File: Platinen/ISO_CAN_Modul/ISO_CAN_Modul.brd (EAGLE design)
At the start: 35.1 x 27.9 mm, 26 parts, among them CON8 Term, IC1 MCP2515-I/P, IC2 ISO1050, IC3 B0505S-1W, X1 8 MHz, X2 Male, X3 Male, X4 Male, X5 AK500/2+M

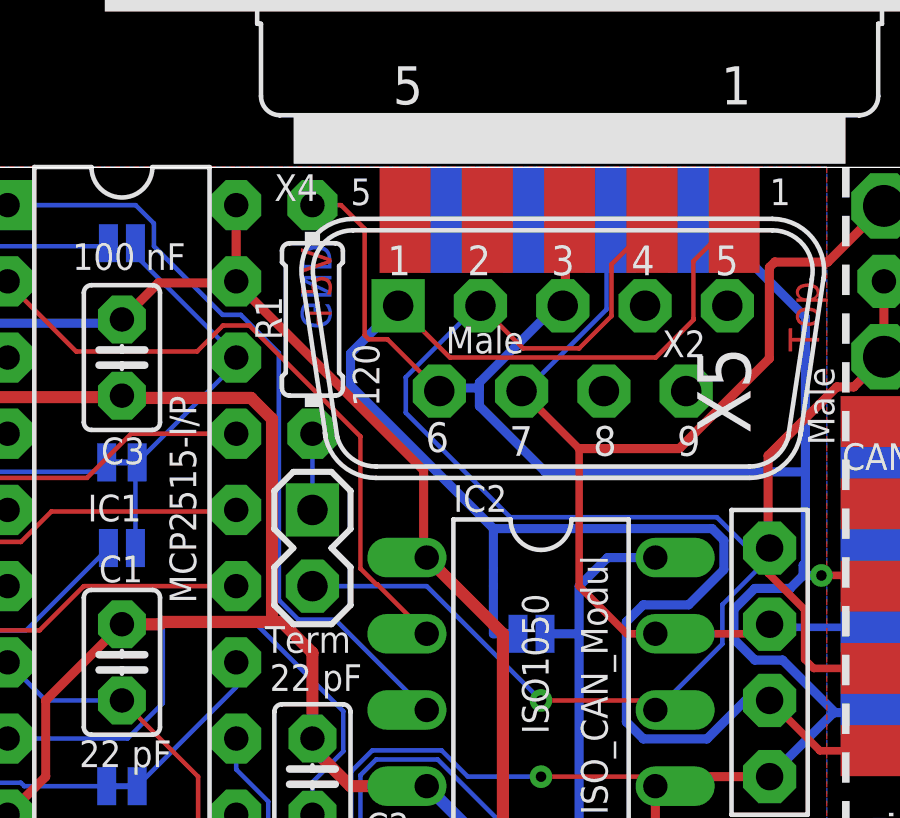
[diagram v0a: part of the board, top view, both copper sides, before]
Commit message: Logo & R1
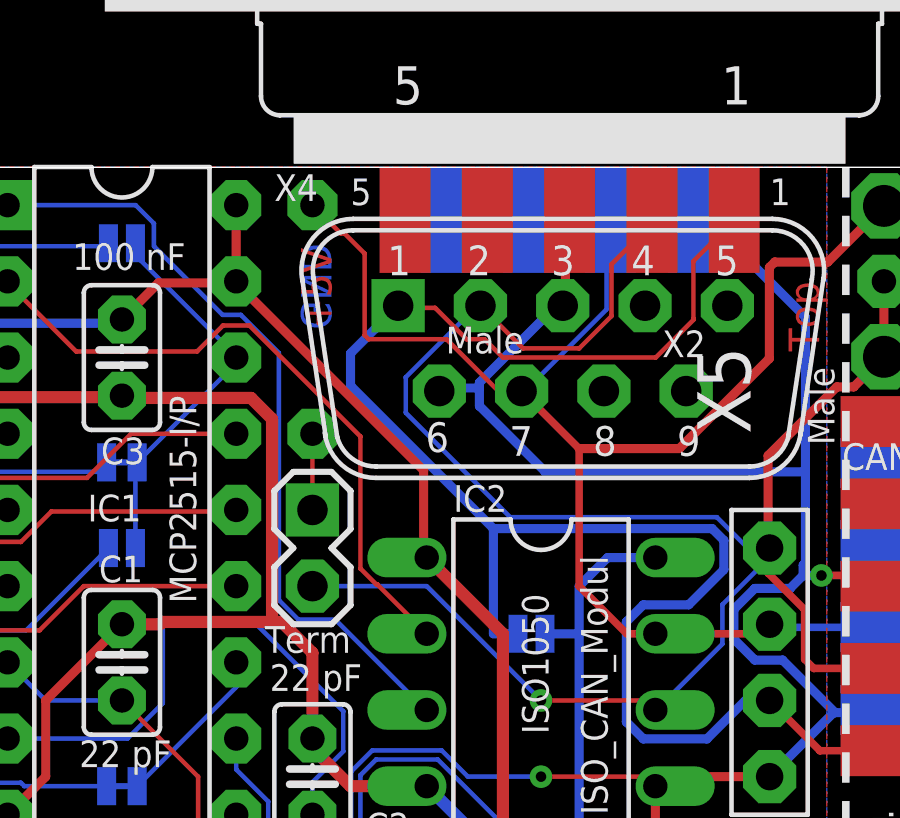
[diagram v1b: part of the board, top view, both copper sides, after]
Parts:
- flipped R1 to the bottom
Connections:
- net CAN_H: now also R1.2
- net GND2: no longer R1.2
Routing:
- net CAN_H: track 40.8 -> 52.0 mm
- net GND2: track 95.2 -> 86.3 mm
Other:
- board text added: "https://wiki.mobaledlib.de"
- board text removed: "https://wiki.mobaledlib.de/doku.php"
